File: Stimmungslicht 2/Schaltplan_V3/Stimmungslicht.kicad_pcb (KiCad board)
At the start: 2 copper layers, 37.8 x 37.8 mm, 19 parts, among them IC1 STM32G031J6M6, J1 Conn_01x01, J2 Conn_01x04_Male, U1 HU2032-LF, U101 Touch_Sens_Pad, U102 Touch_Sens_Pad, U103 Touch_Sens_Pad, U104 Touch_Sens_Pad

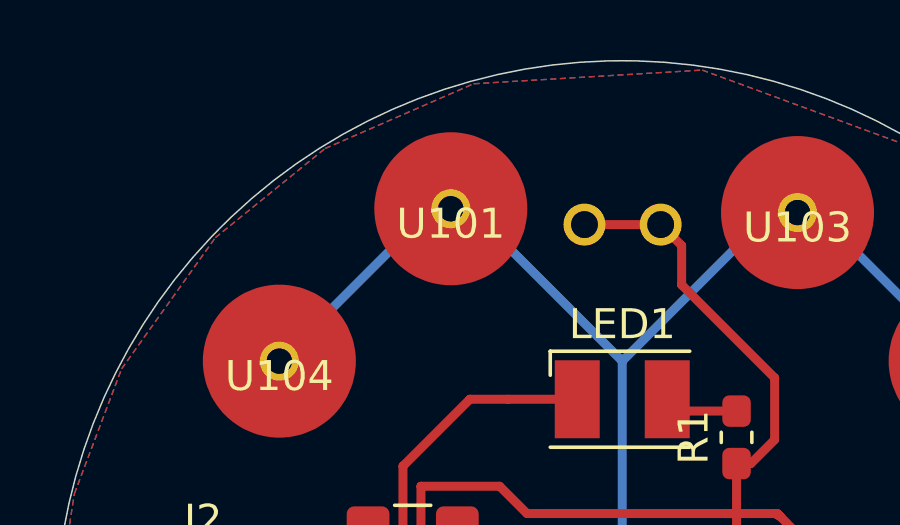
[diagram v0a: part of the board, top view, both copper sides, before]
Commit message: Aktueller Schaltplan
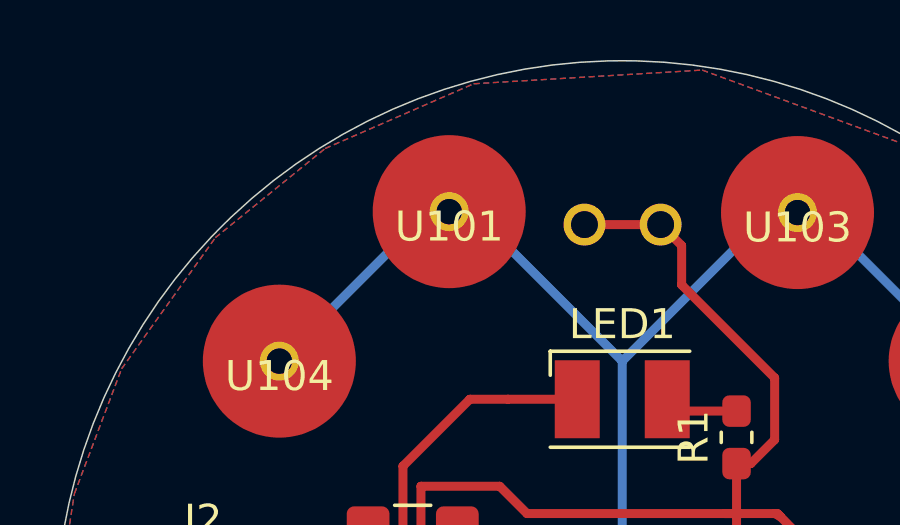
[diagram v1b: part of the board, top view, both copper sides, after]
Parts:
- moved U101 0.11 mm to (138.5, 102.4)
